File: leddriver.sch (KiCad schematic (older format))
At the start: 72 parts, among them J1 CONN_01X01, J2 CONN_01X02, J3 CONN_02X03, J4 USB_OTG, J5 CONN_02X03, J6 CONN_01X04, Q1 Q_NMOS_GDS, Q2 S8050, Q3 S8050, SW1 Rotary_Encoder_Switch, U1 LNK3202/3204-6, U2 ATMEGA328P-AU, U3 HV9910C, U4 PC817, U5 esp8266mod, U6 CH340G, Y1 16MHz, Y2 Crystal

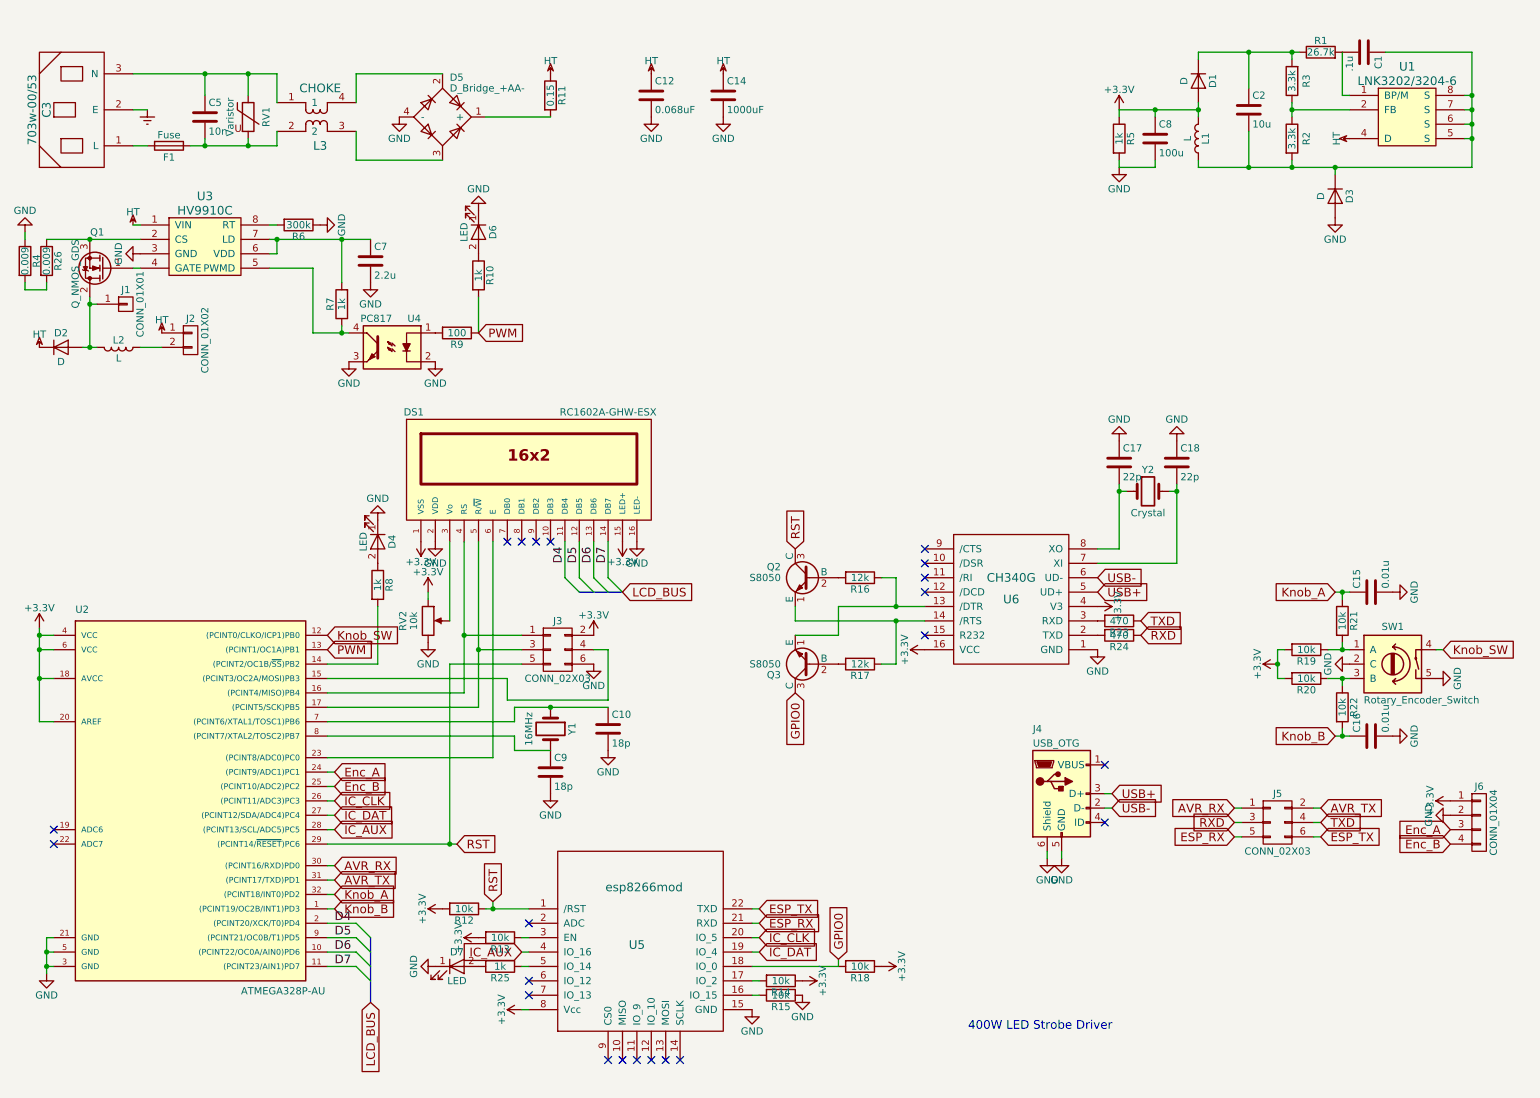
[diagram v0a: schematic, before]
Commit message: PCB
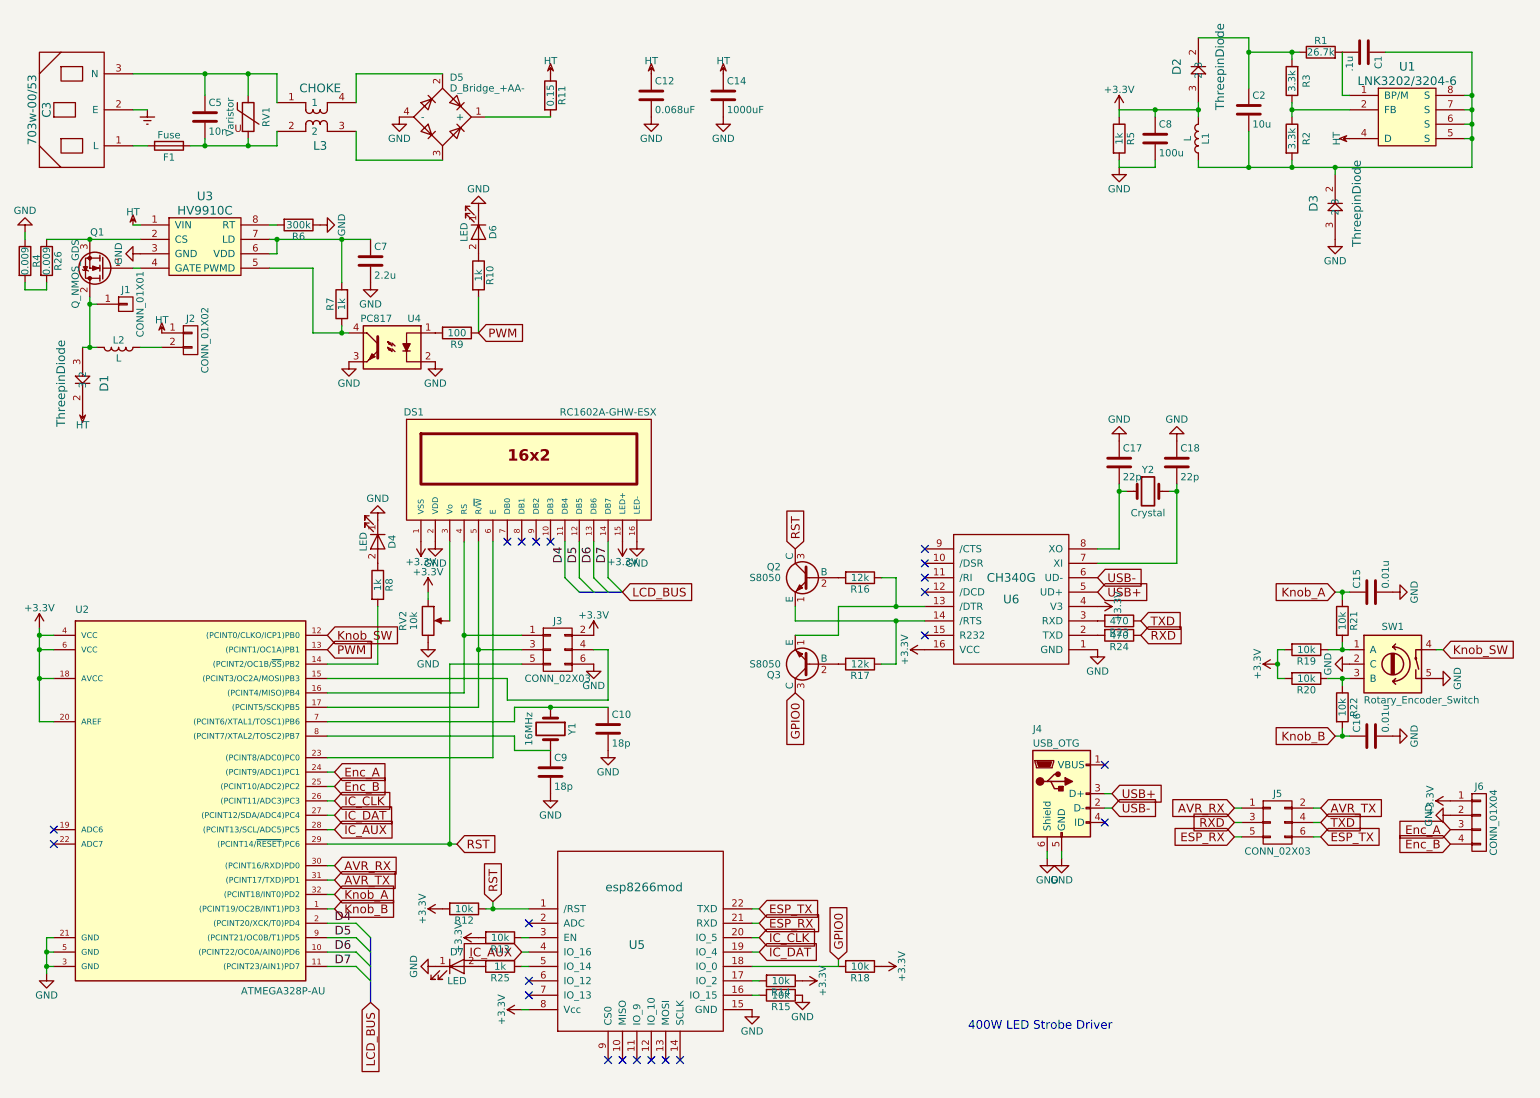
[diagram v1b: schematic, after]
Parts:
- removed D1, D2, D3: D, TO_SOT_Packages_SMD:TO-252-2Lead, symbol D
- added D1, D2, D3: ThreepinDiode, TO_SOT_Packages_SMD:TO-252-2_Rectifier, symbol ThreepinDiode
- C3: footprint (none) -> local_footprints:703w-00-53
- D5: footprint (none) -> local_footprints:ds21221
- J1: footprint (none) -> Connectors:1pin
- L3: footprint (none) -> local_footprints:pm3700
- Q1: footprint TO_SOT_Packages_SMD:TO-252-2Lead -> TO_SOT_Packages_SMD:TO-252-2
- SW1: footprint (none) -> local_footprints:pec12r
- U2: footprint TQFP32 -> Housings_QFP:TQFP-32_7x7mm_Pitch0.8mm
- U5: footprint (none) -> local_footprints:ESP12E
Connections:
- net +3V3: now also D2.3
- net GND: now also D3.3
- net HT: now also D1.2
- net at J1.1 (P1), L2.2, Q1.2 (D): now also D1.3
- net at C1.1, C2.2, L1.1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: now also D3.2
- net at C2.1, R1.1, R3.2: now also D2.2
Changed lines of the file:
@@
 F 0 "C3" H 1100 1250 60  0000 C CNN
 F 1 "703w-00/53" H 1100 1350 60  0000 C CNN
-F 2 "" H 1100 1100 60  0001 C CNN
+F 2 "local_footprints:703w-00-53" H 1100 1100 60  0001 C CNN
 F 3 "" H 1100 1100 60  0001 C CNN
 	1    1100 1100
@@
 F 0 "L3" H 2850 950 60  0000 C CNN
 F 1 "CHOKE" H 2850 1350 60  0000 C CNN
-F 2 "" H 2950 1300 60  0001 C CNN
+F 2 "local_footprints:pm3700" H 2950 1300 60  0001 C CNN
 F 3 "" H 2950 1300 60  0001 C CNN
 	1    2850 1150
@@
 F 0 "D5" H 3750 1425 50  0000 L CNN
 F 1 "D_Bridge_+AA-" H 3750 1350 50  0000 L CNN
-F 2 "" H 3700 1150 50  0001 C CNN
+F 2 "local_footprints:ds21221" H 3700 1150 50  0001 C CNN
 F 3 "" H 3700 1150 50  0001 C CNN
 	1    3700 1150
@@
 F 0 "Q1" H 1350 1950 50  0000 L CNN
 F 1 "Q_NMOS_GDS" V 1550 2000 50  0000 L CNN
-F 2 "TO_SOT_Packages_SMD:TO-252-2Lead" H 1550 2300 50  0001 C CNN
+F 2 "TO_SOT_Packages_SMD:TO-252-2" H 1550 2300 50  0001 C CNN
 F 3 "" H 1350 2200 50  0001 C CNN
 	1    1350 2200
@@
 $EndComp
 $Comp
-L D D2
-U 1 1 5930FC0A
-P 1050 2750
-F 0 "D2" H 1050 2850 50  0000 C CNN
-F 1 "D" H 1050 2650 50  0000 C CNN
-F 2 "TO_SOT_Packages_SMD:TO-252-2Lead" H 1050 2750 50  0001 C CNN
-F 3 "" H 1050 2750 50  0001 C CNN
-	1    1050 2750
-	1    0    0    -1
-$EndComp
-$Comp
 L C C7
 U 1 1 5930FCC5
@@
 F 0 "U2" H 1150 7100 50  0000 L BNN
 F 1 "ATMEGA328P-AU" H 2300 4450 50  0000 L BNN
-F 2 "TQFP32" H 1900 5850 50  0001 C CIN
+F 2 "Housings_QFP:TQFP-32_7x7mm_Pitch0.8mm" H 1900 5850 50  0001 C CIN
 F 3 "" H 1900 5850 50  0001 C CNN
 	1    1900 5850
@@
 F 0 "J1" H 1500 2550 50  0000 C CNN
 F 1 "CONN_01X01" V 1600 2450 50  0000 C CNN
-F 2 "" H 1500 2450 50  0001 C CNN
+F 2 "Connectors:1pin" H 1500 2450 50  0001 C CNN
 F 3 "" H 1500 2450 50  0001 C CNN
 	1    1500 2450
@@
 L HT #PWR03
 U 1 1 59310FDA
-P 900 2750
-F 0 "#PWR03" H 900 2870 50  0001 C CNN
-F 1 "HT" H 900 2840 50  0000 C CNN
-F 2 "" H 900 2750 50  0001 C CNN
-F 3 "" H 900 2750 50  0001 C CNN
-	1    900  2750
-	1    0    0    -1
+P 1200 3200
+F 0 "#PWR03" H 1200 3320 50  0001 C CNN
+F 1 "HT" H 1200 3290 50  0000 C CNN
+F 2 "" H 1200 3200 50  0001 C CNN
+F 3 "" H 1200 3200 50  0001 C CNN
+	1    1200 3200
+	-1   0    0    1
 $EndComp
 $Comp
@@
 $EndComp
 $Comp
-L D D1
-U 1 1 5931592F
-P 8950 900
-F 0 "D1" H 8950 1000 50  0000 C CNN
-F 1 "D" H 8950 800 50  0000 C CNN
-F 2 "TO_SOT_Packages_SMD:TO-252-2Lead" H 8950 900 50  0001 C CNN
-F 3 "" H 8950 900 50  0001 C CNN
-	1    8950 900
-	0    1    1    0
-$EndComp
-$Comp
 L L L1
 U 1 1 59315984
@@
 $EndComp
 $Comp
-L D D3
-U 1 1 593159E9
-P 9900 1700
-F 0 "D3" H 9900 1800 50  0000 C CNN
-F 1 "D" H 9900 1600 50  0000 C CNN
-F 2 "TO_SOT_Packages_SMD:TO-252-2Lead" H 9900 1700 50  0001 C CNN
-F 3 "" H 9900 1700 50  0001 C CNN
-	1    9900 1700
-	0    1    1    0
-$EndComp
-$Comp
 L HT #PWR014
 U 1 1 59318272
@@
 L GND #PWR015
 U 1 1 593254F8
-P 9900 1850
-F 0 "#PWR015" H 9900 1600 50  0001 C CNN
-F 1 "GND" H 9900 1700 50  0000 C CNN
-F 2 "" H 9900 1850 50  0001 C CNN
-F 3 "" H 9900 1850 50  0001 C CNN
-	1    9900 1850
+P 9900 2000
+F 0 "#PWR015" H 9900 1750 50  0001 C CNN
+F 1 "GND" H 9900 1850 50  0000 C CNN
+F 2 "" H 9900 2000 50  0001 C CNN
+F 3 "" H 9900 2000 50  0001 C CNN
+	1    9900 2000
 	1    0    0    -1
 $EndComp
@@
 F 0 "SW1" H 10300 5210 50  0000 C CNN
 F 1 "Rotary_Encoder_Switch" H 10500 4700 50  0000 C CNN
-F 2 "" H 10200 5110 50  0001 C CNN
+F 2 "local_footprints:pec12r" H 10200 5110 50  0001 C CNN
 F 3 "" H 10300 5210 50  0001 C CNN
 	1    10300 4950
@@
 F 0 "U5" H 5050 6900 60  0000 C CNN
 F 1 "esp8266mod" H 5100 7300 60  0000 C CNN
-F 2 "" H 5050 5900 60  0001 C CNN
+F 2 "local_footprints:ESP12E" H 5050 5900 60  0001 C CNN
 F 3 "" H 5050 5900 60  0001 C CNN
 	1    5050 6900
@@
 	10850 700  10250 700
 Wire Wire Line
-	9650 700  8950 700
-Wire Wire Line
-	8950 700  8950 750
-Wire Wire Line
 	9600 750  9600 700
 Connection ~ 9600 700
 Wire Wire Line
-	9300 950  9300 700
+	9300 600  9300 950
 Connection ~ 9300 700
 Wire Wire Line
@@
 Wire Wire Line
 	800  1950 800  2000
+$Comp
+L ThreepinDiode D1
+U 1 1 593216F7
+P 1350 3000
+F 0 "D1" H 1350 3000 60  0000 C CNN
+F 1 "ThreepinDiode" H 1350 3300 60  0000 C CNN
+F 2 "TO_SOT_Packages_SMD:TO-252-2_Rectifier" H 1350 3000 60  0001 C CNN
+F 3 "" H 1350 3000 60  0001 C CNN
+	1    1350 3000
+	0    -1   -1   0
+$EndComp
+$Comp
+L ThreepinDiode D3
+U 1 1 5932423A
+P 9750 1750
+F 0 "D3" H 9750 1750 60  0000 C CNN
+F 1 "ThreepinDiode" H 9750 2050 60  0000 C CNN
+F 2 "TO_SOT_Packages_SMD:TO-252-2_Rectifier" H 9750 1750 60  0001 C CNN
+F 3 "" H 9750 1750 60  0001 C CNN
+	1    9750 1750
+	0    1    1    0
+$EndComp
+$Comp
+L ThreepinDiode D2
+U 1 1 59324B9B
+P 8800 800
+F 0 "D2" H 8800 800 60  0000 C CNN
+F 1 "ThreepinDiode" H 8800 1100 60  0000 C CNN
+F 2 "TO_SOT_Packages_SMD:TO-252-2_Rectifier" H 8800 800 60  0001 C CNN
+F 3 "" H 8800 800 60  0001 C CNN
+	1    8800 800
+	0    1    1    0
+$EndComp
+Wire Wire Line
+	8950 600  9300 600
+Wire Wire Line
+	9300 700  9650 700
 $EndSCHEMATC
